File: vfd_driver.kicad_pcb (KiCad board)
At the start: 2 copper layers, 181.6 x 48.3 mm, 44 parts, among them CON1 AVR-ISP-6, J1 PWR, J2 Display, J6 MH, J7 MH, J8 MH, J9 MH, U1 ATTINY2313-20SU, U10 74HC595, U11 74HC595, U12 74HC595, U13 74HC595, U14 ULN2803A, U15 ULN2803A, U16 ULN2003, U17 ULN2003, U18 LM1117-3.3, U19 LT1073, U2 74HC595, U3 74HC595, U4 74HC595, U5 74HC595, U6 ULN2803A, U7 ULN2003, U8 ULN2003, U9 ULN2003

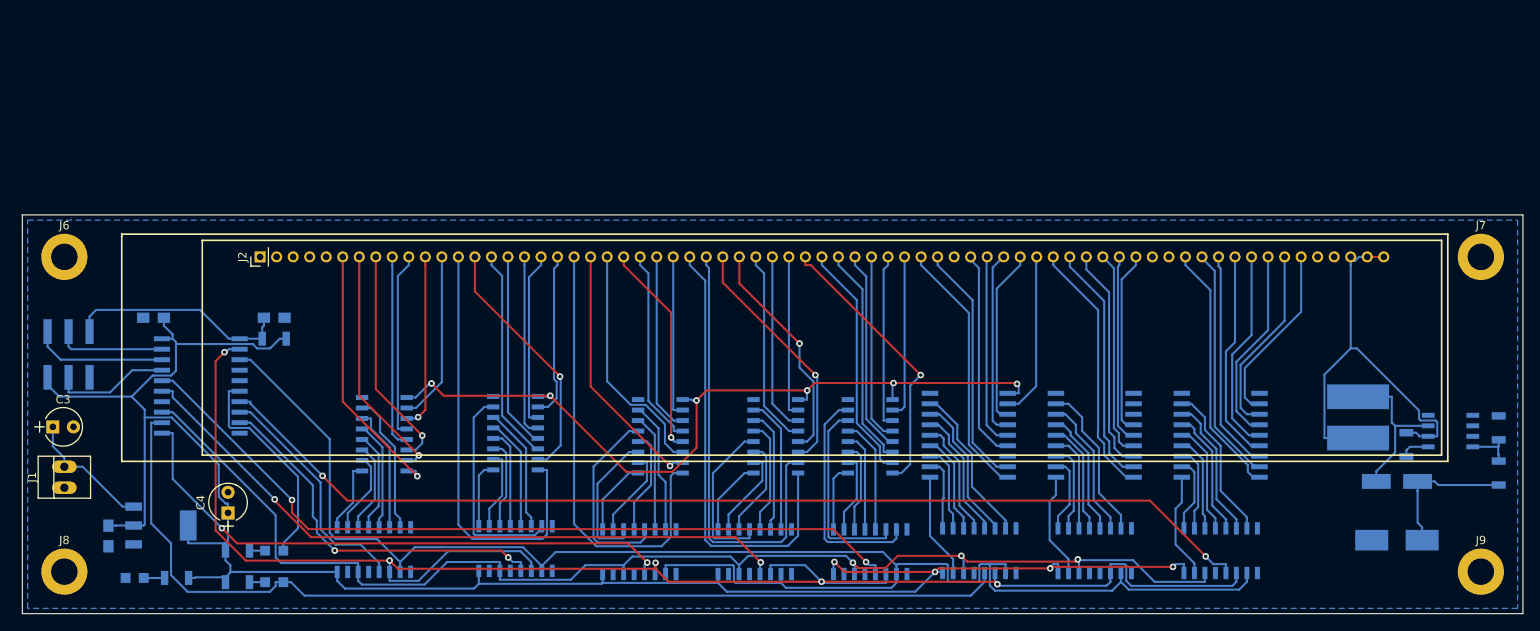
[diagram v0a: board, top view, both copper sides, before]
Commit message: first version
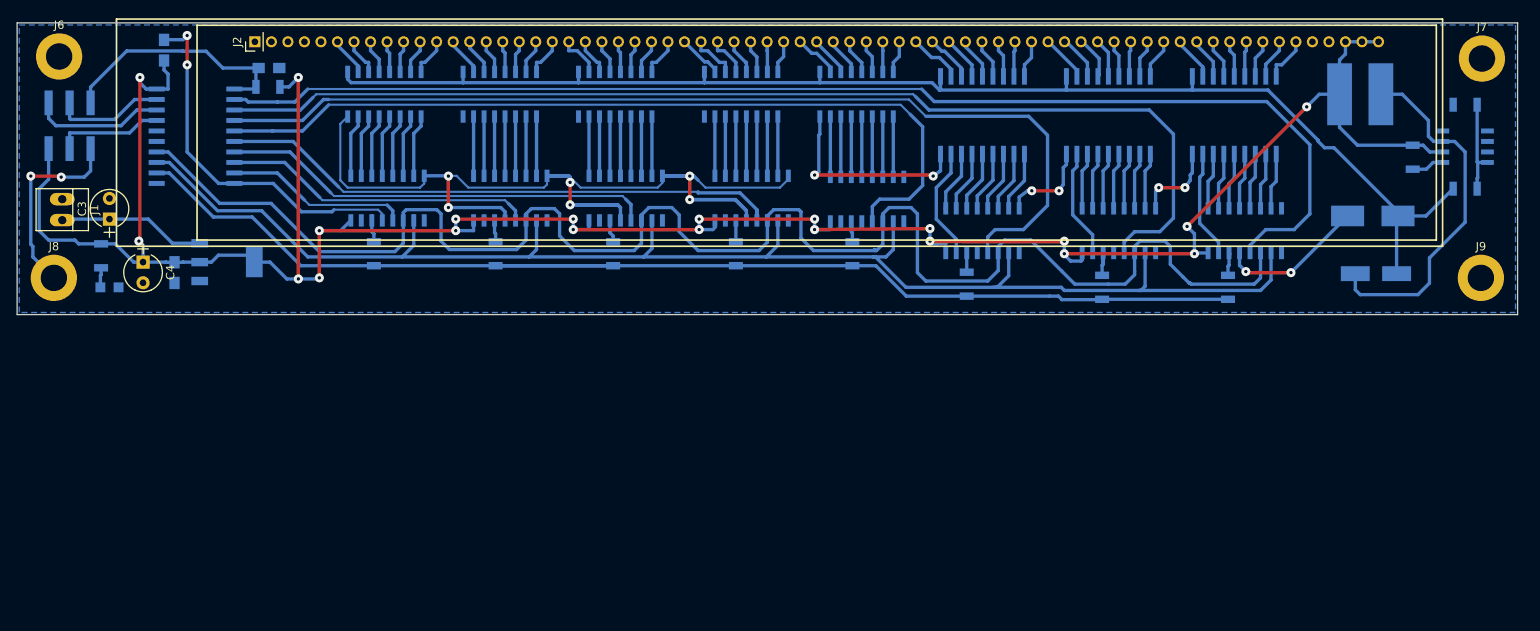
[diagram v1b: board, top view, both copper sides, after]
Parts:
- removed D3, D4: LED, LEDs:LED_0805
- removed R6, R7: 470, Resistors_SMD:R_1206
- added R10: 0, Resistors_SMD:R_1206, B.Cu at (72.5, 46.6)
- added R11: 0, Resistors_SMD:R_1206, B.Cu at (101.6, 46.6)
- added R12: 0, Resistors_SMD:R_1206, B.Cu at (145.9, 50.7)
- added R13: 0, Resistors_SMD:R_1206, B.Cu at (161.2, 50.7)
- added R14: 0, Resistors_SMD:R_1206, B.Cu at (86.7, 46.6)
- added R15: 0, Resistors_SMD:R_1206, B.Cu at (115.7, 46.6)
- added R8: 0, Resistors_SMD:R_1206, B.Cu at (129.5, 50.3)
- added R9: 0, Resistors_SMD:R_1206, B.Cu at (57.8, 46.6)
- moved U12 42.8 mm to (88.3, 39.9)
- moved U5 42.8 mm to (103.5, 39.9)
- moved U13 42.7 mm to (117.5, 40.0)
- moved U3 42.6 mm to (59.4, 39.9)
- moved U4 42.4 mm to (74.3, 39.9)
- moved U16 41.8 mm to (87.0, 27.3), turned to 90 degrees
- moved U9 41.6 mm to (102.2, 27.3), turned to 90 degrees
- moved U17 41.4 mm to (116.2, 27.3), turned to 90 degrees
- moved U7 41.1 mm to (59.1, 27.3), turned to 90 degrees
- moved U8 41.1 mm to (73.0, 27.3), turned to 90 degrees
- moved R5 40.0 mm to (24.8, 46.9), turned to 270 degrees
- moved C6 39.4 mm to (178.7, 42.0)
- moved R4 39.3 mm to (189.9, 28.6), turned to 180 degrees
- moved L1 39.1 mm to (177.2, 27.3), turned to 0 degrees
- moved U10 38.8 mm to (148.0, 43.8)
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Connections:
- J2 pad 27: /L41 -> /L47
- J2 pad 28: /L42 -> /L46
- J2 pad 29: /L43 -> /L45
- J2 pad 31: /L45 -> /L43
- J2 pad 32: /L46 -> /L42
- J2 pad 33: /L47 -> /L41
- U1 pad 11: /RCLK_5 -> (no net)
- U1 pad 12: /RCLK_0 -> /SER
- U1 pad 13: /SER -> /SRCLR
- U1 pad 14: (no net) -> /SRCLK
- U1 pad 15: /RCLK_6 -> (no net)
- U1 pad 16: /RCLK_7 -> (no net)
- U1 pad 2: /SRCLK -> /RCLK_2
- U1 pad 3: /SRCLR -> /RCLK_1
- U1 pad 4: (no net) -> /RCLK_0
- U1 pad 5: (no net) -> /RCLK_7
- U1 pad 6: /RCLK_1 -> /RCLK_6
- U1 pad 7: /RCLK_2 -> /RCLK_5
- U1 pad 8: /RCLK_3 -> /RCLK_4
- U1 pad 9: /RCLK_4 -> /RCLK_3
- U10 pad 14: /SER -> Net-(R12-Pad1)
- U11 pad 14: /SER -> Net-(R13-Pad1)
- U12 pad 14: /SER -> Net-(R14-Pad1)
- U13 pad 14: /SER -> Net-(R15-Pad1)
- U14 pad 1: Net-(U10-Pad15) -> Net-(U10-Pad7)
- U14 pad 11: /G28 -> /G21
- U14 pad 12: /G27 -> /G22
- U14 pad 13: /G26 -> /G23
- U14 pad 14: /G25 -> /G24
- U14 pad 15: /G24 -> /G25
- U14 pad 16: /G23 -> /G26
- U14 pad 17: /G22 -> /G27
- U14 pad 18: /G21 -> /G28
- U14 pad 2: Net-(U10-Pad1) -> Net-(U10-Pad6)
- U14 pad 3: Net-(U10-Pad2) -> Net-(U10-Pad5)
- U14 pad 4: Net-(U10-Pad3) -> Net-(U10-Pad4)
- U14 pad 5: Net-(U10-Pad4) -> Net-(U10-Pad3)
- U14 pad 6: Net-(U10-Pad5) -> Net-(U10-Pad2)
- U14 pad 7: Net-(U10-Pad6) -> Net-(U10-Pad1)
- U14 pad 8: Net-(U10-Pad7) -> Net-(U10-Pad15)
- U15 pad 1: Net-(U11-Pad15) -> Net-(U11-Pad7)
- U15 pad 11: /G38 -> /G31
- U15 pad 12: /G37 -> /G32
- U15 pad 13: /G36 -> /G33
- U15 pad 14: /G35 -> /G34
- U15 pad 15: /G34 -> /G35
- U15 pad 16: /G33 -> /G36
- U15 pad 17: /G32 -> /G37
- U15 pad 18: /G31 -> /G38
- U15 pad 2: Net-(U11-Pad1) -> Net-(U11-Pad6)
- U15 pad 3: Net-(U11-Pad2) -> Net-(U11-Pad5)
- U15 pad 4: Net-(U11-Pad3) -> Net-(U11-Pad4)
- U15 pad 5: Net-(U11-Pad4) -> Net-(U11-Pad3)
- U15 pad 6: Net-(U11-Pad5) -> Net-(U11-Pad2)
- U15 pad 7: Net-(U11-Pad6) -> Net-(U11-Pad1)
- U15 pad 8: Net-(U11-Pad7) -> Net-(U11-Pad15)
- U16 pad 1: Net-(U12-Pad1) -> Net-(U12-Pad7)
- U16 pad 10: /L37 -> /L31
- U16 pad 11: /L36 -> /L32
- U16 pad 12: /L35 -> /L33
- U16 pad 14: /L33 -> /L35
- U16 pad 15: /L32 -> /L36
- U16 pad 16: /L31 -> /L37
- U16 pad 2: Net-(U12-Pad2) -> Net-(U12-Pad6)
- U16 pad 3: Net-(U12-Pad3) -> Net-(U12-Pad5)
- U16 pad 5: Net-(U12-Pad5) -> Net-(U12-Pad3)
- U16 pad 6: Net-(U12-Pad6) -> Net-(U12-Pad2)
- U16 pad 7: Net-(U12-Pad7) -> Net-(U12-Pad1)
- U17 pad 1: Net-(U13-Pad1) -> Net-(U13-Pad7)
- U17 pad 10: /L57 -> /L51
- U17 pad 11: /L56 -> /L52
- U17 pad 12: /L55 -> /L53
- U17 pad 14: /L53 -> /L55
- U17 pad 15: /L52 -> /L56
- U17 pad 16: /L51 -> /L57
- U17 pad 2: Net-(U13-Pad2) -> Net-(U13-Pad6)
- U17 pad 3: Net-(U13-Pad3) -> Net-(U13-Pad5)
- U17 pad 5: Net-(U13-Pad5) -> Net-(U13-Pad3)
- U17 pad 6: Net-(U13-Pad6) -> Net-(U13-Pad2)
- U17 pad 7: Net-(U13-Pad7) -> Net-(U13-Pad1)
- U2 pad 14: /SER -> Net-(R8-Pad1)
- U3 pad 14: /SER -> Net-(R9-Pad1)
- U4 pad 14: /SER -> Net-(R10-Pad1)
- U5 pad 14: /SER -> Net-(R11-Pad1)
- U6 pad 1: Net-(U2-Pad15) -> Net-(U2-Pad7)
- U6 pad 11: /G18 -> /G11
- U6 pad 12: /G17 -> /G12
- U6 pad 13: /G16 -> /G13
- U6 pad 14: /G15 -> /G14
- U6 pad 15: /G14 -> /G15
- U6 pad 16: /G13 -> /G16
- U6 pad 17: /G12 -> /G17
- U6 pad 18: /G11 -> /G18
- U6 pad 2: Net-(U2-Pad1) -> Net-(U2-Pad6)
- U6 pad 3: Net-(U2-Pad2) -> Net-(U2-Pad5)
- U6 pad 4: Net-(U2-Pad3) -> Net-(U2-Pad4)
- U6 pad 5: Net-(U2-Pad4) -> Net-(U2-Pad3)
- U6 pad 6: Net-(U2-Pad5) -> Net-(U2-Pad2)
- U6 pad 7: Net-(U2-Pad6) -> Net-(U2-Pad1)
- U6 pad 8: Net-(U2-Pad7) -> Net-(U2-Pad15)
- U7 pad 1: Net-(U3-Pad1) -> Net-(U3-Pad7)
- U7 pad 10: /L17 -> /L11
- U7 pad 11: /L16 -> /L12
- U7 pad 12: /L15 -> /L13
- U7 pad 14: /L13 -> /L15
- U7 pad 15: /L12 -> /L16
- U7 pad 16: /L11 -> /L17
- U7 pad 2: Net-(U3-Pad2) -> Net-(U3-Pad6)
- U7 pad 3: Net-(U3-Pad3) -> Net-(U3-Pad5)
- U7 pad 5: Net-(U3-Pad5) -> Net-(U3-Pad3)
- U7 pad 6: Net-(U3-Pad6) -> Net-(U3-Pad2)
- U7 pad 7: Net-(U3-Pad7) -> Net-(U3-Pad1)
- U8 pad 1: Net-(U4-Pad1) -> Net-(U4-Pad7)
- U8 pad 10: /L27 -> /L21
- U8 pad 11: /L26 -> /L22
- U8 pad 12: /L25 -> /L23
- U8 pad 14: /L23 -> /L25
- U8 pad 15: /L22 -> /L26
- U8 pad 16: /L21 -> /L27
- U8 pad 2: Net-(U4-Pad2) -> Net-(U4-Pad6)
- U8 pad 3: Net-(U4-Pad3) -> Net-(U4-Pad5)
- U8 pad 5: Net-(U4-Pad5) -> Net-(U4-Pad3)
- U8 pad 6: Net-(U4-Pad6) -> Net-(U4-Pad2)
- U8 pad 7: Net-(U4-Pad7) -> Net-(U4-Pad1)
- U9 pad 1: Net-(U5-Pad1) -> Net-(U5-Pad7)
- U9 pad 2: Net-(U5-Pad2) -> Net-(U5-Pad6)
- U9 pad 3: Net-(U5-Pad3) -> Net-(U5-Pad5)
- U9 pad 5: Net-(U5-Pad5) -> Net-(U5-Pad3)
- U9 pad 6: Net-(U5-Pad6) -> Net-(U5-Pad2)
- U9 pad 7: Net-(U5-Pad7) -> Net-(U5-Pad1)
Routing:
- net GND: track 0.00 -> 263.7 mm, vias 0 -> 18
- net /RCLK_1: track 26.1 -> 135.1 mm
- net /L41: track 54.7 -> 3.94 mm
- net /L42: track 54.2 -> 3.66 mm
- net /L31: track 54.6 -> 5.26 mm
- net /L21: track 53.0 -> 4.67 mm
- net +36V: track 114.3 -> 161.6 mm, vias 6 -> 0
- net /L51: track 34.4 -> 5.80 mm, vias 1 -> 0
- net /L11: track 32.1 -> 4.69 mm, vias 1 -> 0
- net /L32: track 31.0 -> 4.53 mm, vias 1 -> 0
- net /L22: track 30.6 -> 4.37 mm, vias 1 -> 0
- net /L43: track 29.9 -> 3.97 mm, vias 1 -> 0
- net /G21: track 31.3 -> 5.68 mm
- net /G31: track 30.9 -> 5.32 mm
- net /G32: track 30.3 -> 5.02 mm
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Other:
- board size 181.6 x 48.3 mm -> 181.6 x 35.3 mm
- net class Default: trace_width 0.25 -> 0.254
- net class signal added: clearance 0.2, trace_width 0.4064, via_dia 1.1, via_drill 0.4
